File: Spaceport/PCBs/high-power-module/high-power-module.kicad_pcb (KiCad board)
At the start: 4 copper layers, 37.4 x 37.6 mm, 77 parts, among them J1 Conn_01x06_Pin, J2 SMA, J3 Conn_01x06_Pin, J4 Conn_01x02_Pin, U1 Si4463, U2 SN74LV1T08QDBVRQ1, U3 TPS62177DQCR

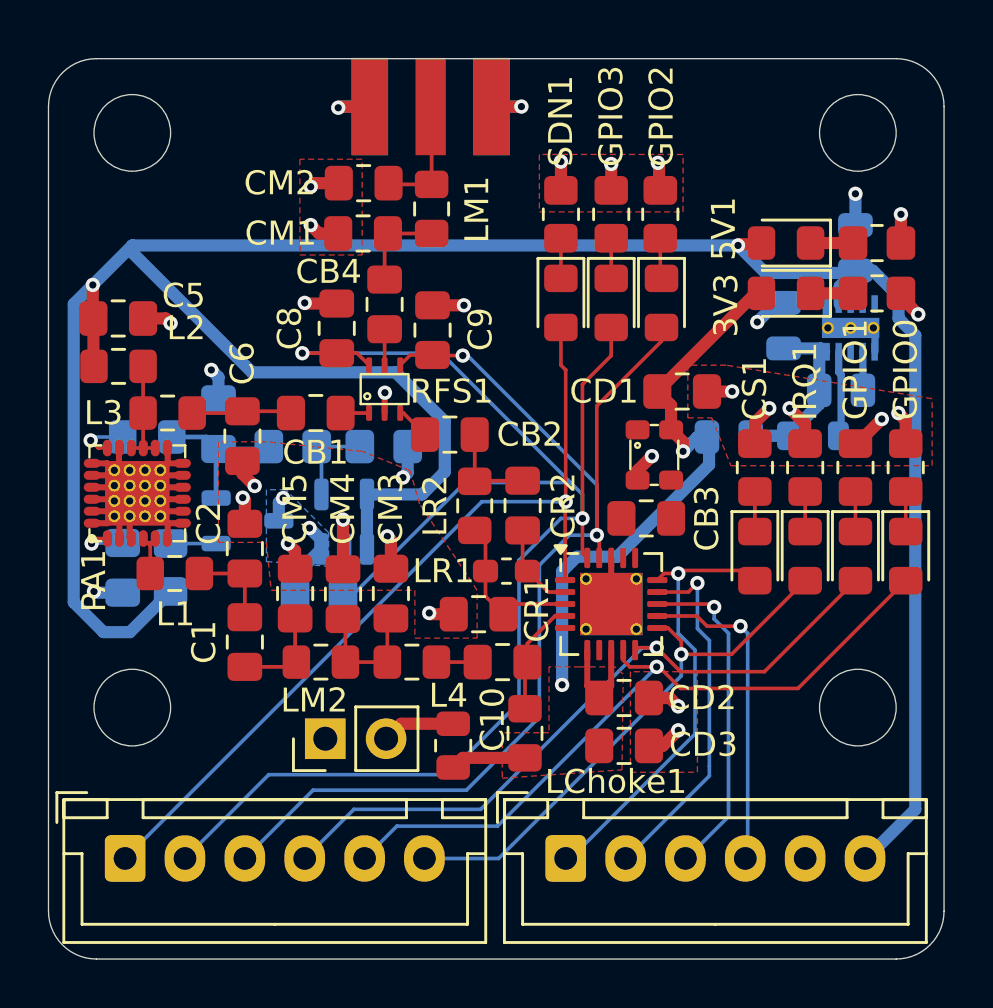
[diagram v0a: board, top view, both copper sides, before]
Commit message: add screw holes to HPM paste layer
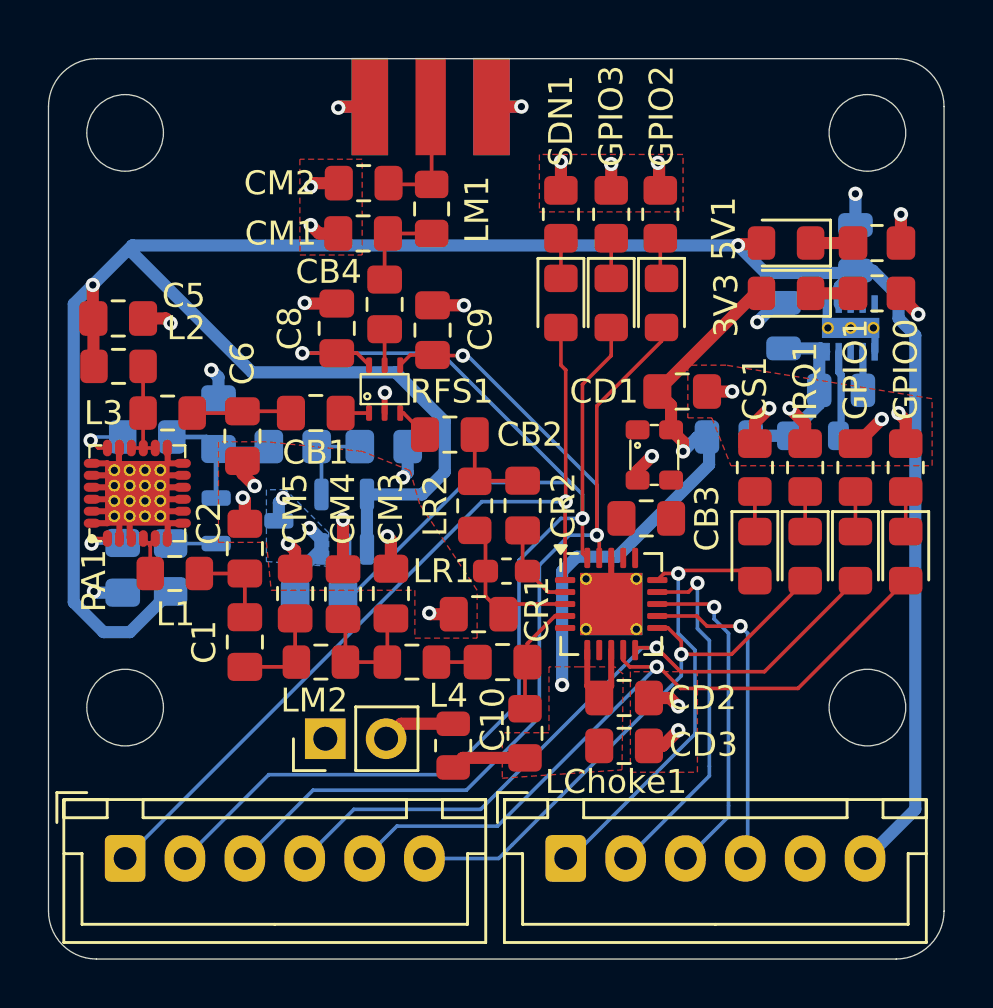
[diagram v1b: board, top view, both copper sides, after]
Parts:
- moved H2 0.40 mm to (158.9, 73.5)
- moved H3 0.40 mm to (158.9, 97.5)
- moved H1 0.30 mm to (127.9, 73.5)
- moved H4 0.30 mm to (127.9, 97.5)
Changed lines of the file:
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@@
 	(footprint "MountingHole:MountingHole_3.2mm_M3"
 		(layer "F.Cu")
-		(at 128.2 97.5)
+		(at 127.9 97.5)
 		(descr "Mounting Hole 3.2mm, no annular, M3")
 		(tags "mounting hole 3.2mm no annular m3")
@@
 			(size 3.2 3.2)
 			(drill 3.2)
-			(layers "*.Cu" "*.Mask")
+			(layers "F&B.Cu" "*.Paste" "*.Mask")
 		)
 	)
@@
 	(footprint "MountingHole:MountingHole_3.2mm_M3"
 		(layer "F.Cu")
-		(at 128.2 73.5)
+		(at 127.9 73.5)
 		(descr "Mounting Hole 3.2mm, no annular, M3")
 		(tags "mounting hole 3.2mm no annular m3")
@@
 			(size 3.2 3.2)
 			(drill 3.2)
-			(layers "*.Cu" "*.Mask")
+			(layers "F&B.Cu" "*.Paste" "*.Mask")
 		)
 	)
@@
 	(footprint "MountingHole:MountingHole_3.2mm_M3"
 		(layer "F.Cu")
-		(at 158.5 73.5)
+		(at 158.9 73.5)
 		(descr "Mounting Hole 3.2mm, no annular, M3")
 		(tags "mounting hole 3.2mm no annular m3")
@@
 			(size 3.2 3.2)
 			(drill 3.2)
-			(layers "*.Cu" "*.Mask")
+			(layers "F&B.Cu" "*.Paste" "*.Mask")
 		)
 	)
 	(footprint "MountingHole:MountingHole_3.2mm_M3"
 		(layer "F.Cu")
-		(at 158.5 97.5)
+		(at 158.9 97.5)
 		(descr "Mounting Hole 3.2mm, no annular, M3")
 		(tags "mounting hole 3.2mm no annular m3")
@@
 			(size 3.2 3.2)
 			(drill 3.2)
-			(layers "*.Cu" "*.Mask")
+			(layers "F&B.Cu" "*.Paste" "*.Mask")
 		)
 	)
